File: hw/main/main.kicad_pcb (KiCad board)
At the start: 2 copper layers, 50 x 50 mm, 22 parts, among them U1 MCP1703A-3302, U2 STM32L011D3, X1 01x04_P2.54mm_Hor, X2 01x04_P2.54mm_Hor

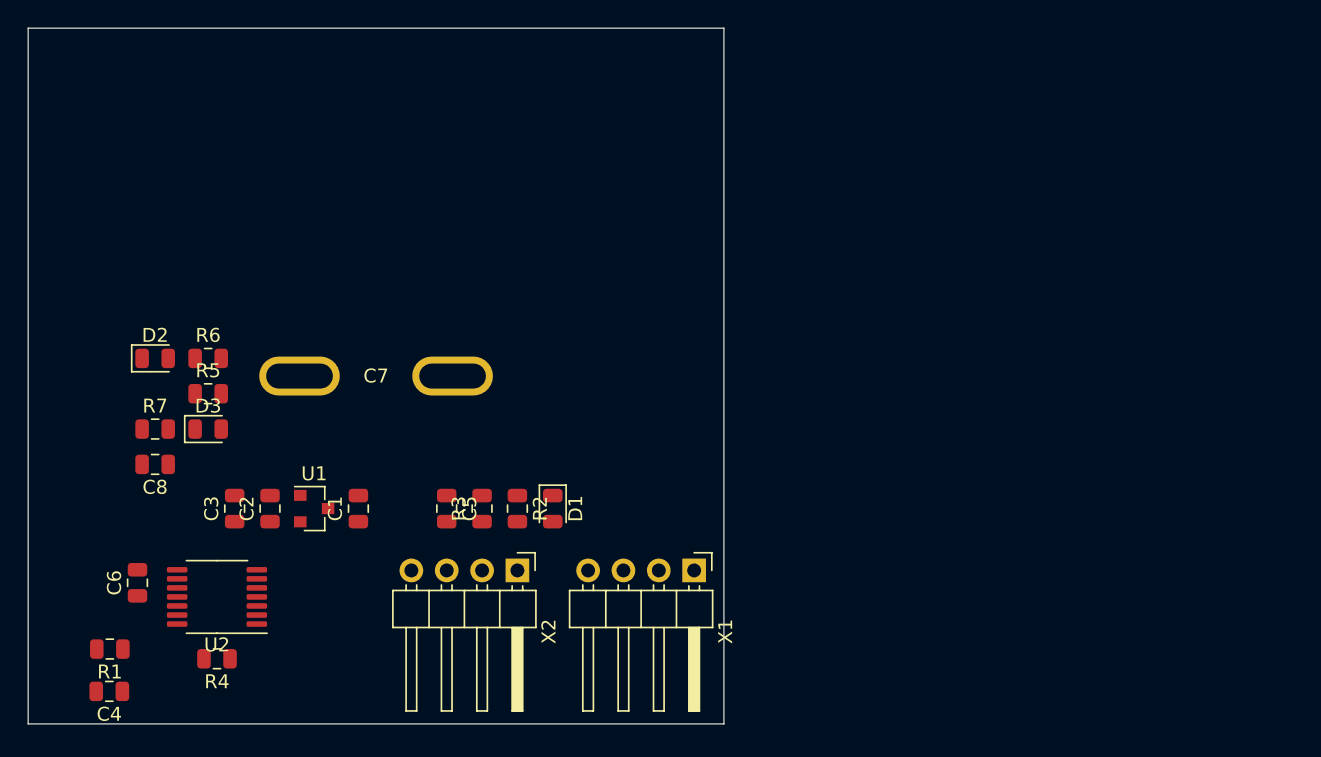
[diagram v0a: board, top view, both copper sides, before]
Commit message: wip
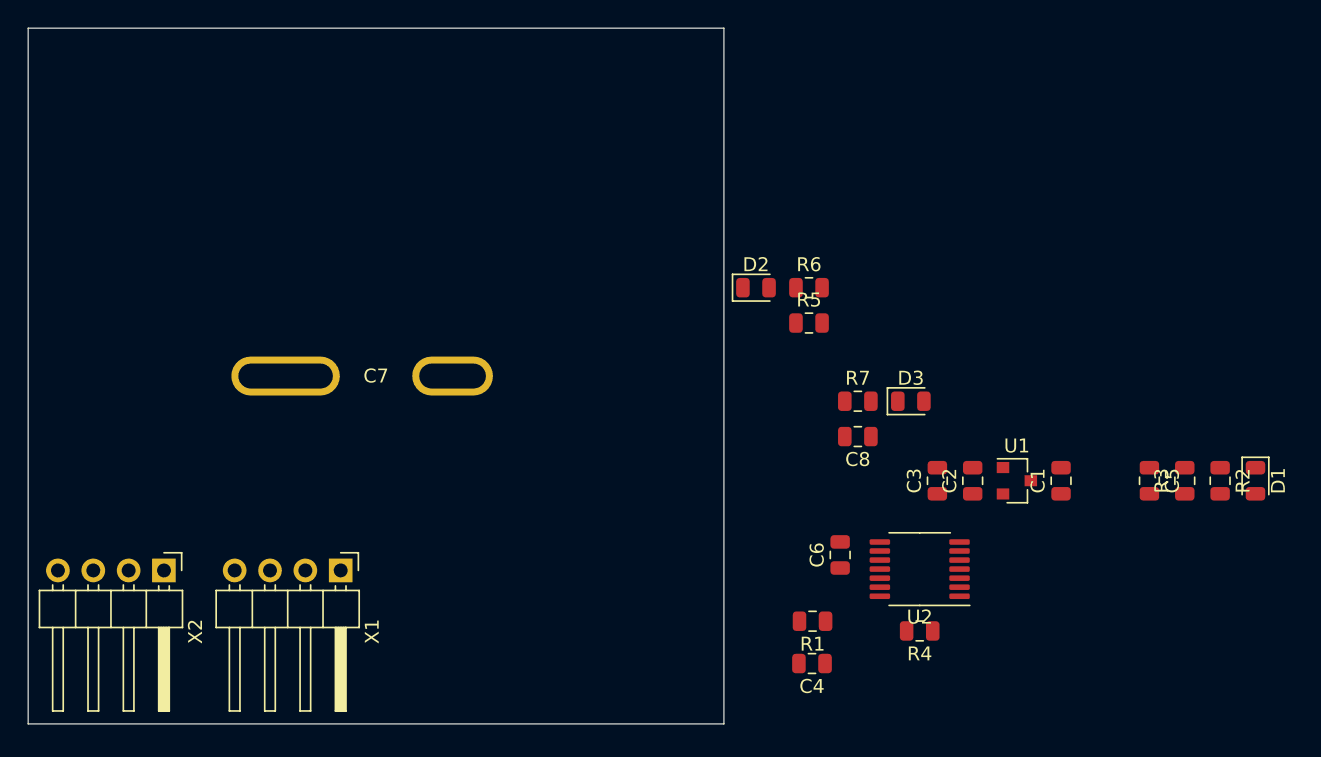
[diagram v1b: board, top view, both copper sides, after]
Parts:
- moved C1 50.5 mm to (199.2, 102.5)
- moved C2 50.5 mm to (192.9, 102.5)
- moved C3 50.5 mm to (190.3, 102.5)
- moved C4 50.5 mm to (181.3, 115.7)
- moved C5 50.5 mm to (205.6, 102.5)
- moved C6 50.5 mm to (183.4, 107.9)
- moved C8 50.5 mm to (184.6, 99.3)
- moved D1 50.5 mm to (213.2, 102.5)
- moved D3 50.5 mm to (188.4, 96.8)
- moved R1 50.5 mm to (181.4, 112.6)
- moved R2 50.5 mm to (210.7, 102.5)
- moved R3 50.5 mm to (208.1, 102.5)
- moved R4 50.5 mm to (189.1, 113.3)
- moved R7 50.5 mm to (184.6, 96.8)
- moved U1 50.5 mm to (196.1, 102.5)
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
